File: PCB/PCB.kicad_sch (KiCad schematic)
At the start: 3 parts, among them J1 TFT Display, J2 PowerBoost 500c, U1 Pico

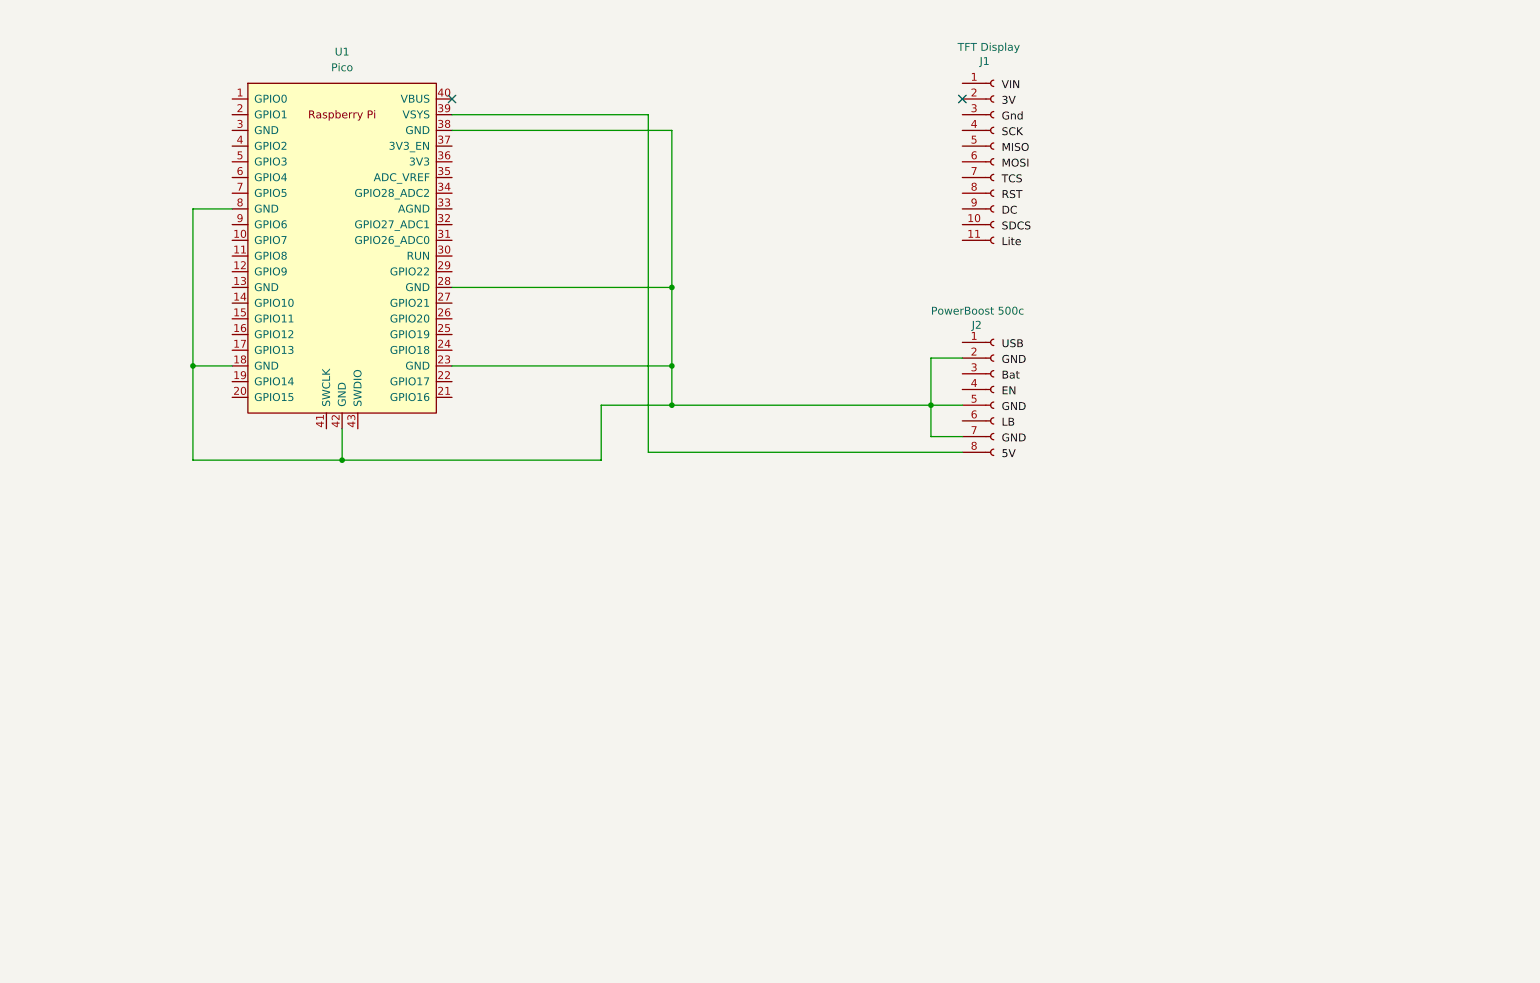
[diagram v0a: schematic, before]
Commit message: Finished controller schematic and mostly finished pcb
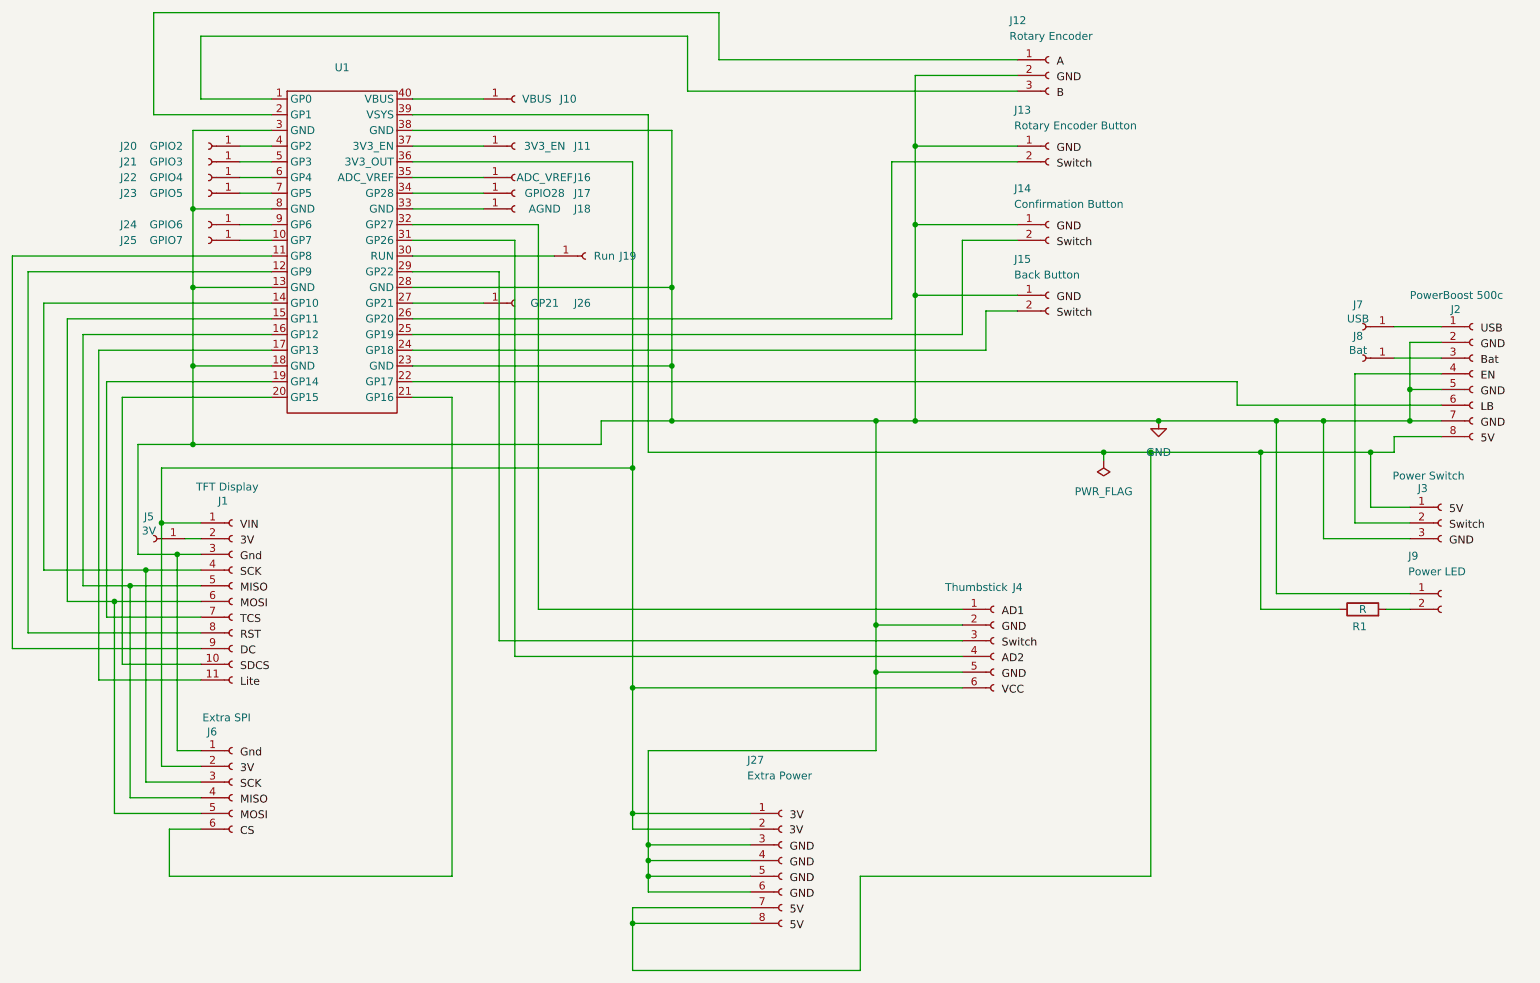
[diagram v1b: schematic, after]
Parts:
- removed U1: Pico, RPi_Pico:RPi_Pico_SMD_TH, symbol RPi_Pico:Pico
- added J10: VBUS, Connector_PinHeader_2.54mm:PinHeader_1x01_P2.54mm_Vertical, symbol Connector:Conn_01x01_Socket
- added J11: 3V3_EN, Connector_PinHeader_2.54mm:PinHeader_1x01_P2.54mm_Vertical, symbol Connector:Conn_01x01_Socket
- added J12: Rotary Encoder, Connector_PinHeader_2.54mm:PinHeader_1x03_P2.54mm_Vertical, symbol Connector:Conn_01x03_Socket
- added J13: Rotary Encoder Button, Connector_PinHeader_2.54mm:PinHeader_1x02_P2.54mm_Vertical, symbol Connector:Conn_01x02_Socket
- added J14: Confirmation Button, Connector_PinHeader_2.54mm:PinHeader_1x02_P2.54mm_Vertical, symbol Connector:Conn_01x02_Socket
- added J15: Back Button, Connector_PinHeader_2.54mm:PinHeader_1x02_P2.54mm_Vertical, symbol Connector:Conn_01x02_Socket
- added J16: ADC_VREF, Connector_PinHeader_2.54mm:PinHeader_1x01_P2.54mm_Vertical, symbol Connector:Conn_01x01_Socket
- added J17: GPIO28, Connector_PinHeader_2.54mm:PinHeader_1x01_P2.54mm_Vertical, symbol Connector:Conn_01x01_Socket
- added J18: AGND, Connector_PinHeader_2.54mm:PinHeader_1x01_P2.54mm_Vertical, symbol Connector:Conn_01x01_Socket
- added J19: Run, Connector_PinHeader_2.54mm:PinHeader_1x01_P2.54mm_Vertical, symbol Connector:Conn_01x01_Socket
- added J20: GPIO2, Connector_PinHeader_2.54mm:PinHeader_1x01_P2.54mm_Vertical, symbol Connector:Conn_01x01_Socket
- added J21: GPIO3, Connector_PinHeader_2.54mm:PinHeader_1x01_P2.54mm_Vertical, symbol Connector:Conn_01x01_Socket
- added J22: GPIO4, Connector_PinHeader_2.54mm:PinHeader_1x01_P2.54mm_Vertical, symbol Connector:Conn_01x01_Socket
- added J23: GPIO5, Connector_PinHeader_2.54mm:PinHeader_1x01_P2.54mm_Vertical, symbol Connector:Conn_01x01_Socket
- added J24: GPIO6, Connector_PinHeader_2.54mm:PinHeader_1x01_P2.54mm_Vertical, symbol Connector:Conn_01x01_Socket
- added J25: GPIO7, Connector_PinHeader_2.54mm:PinHeader_1x01_P2.54mm_Vertical, symbol Connector:Conn_01x01_Socket
- added J26: GP21, Connector_PinHeader_2.54mm:PinHeader_1x01_P2.54mm_Vertical, symbol Connector:Conn_01x01_Socket
- added J27: Extra Power, Connector_PinHeader_2.54mm:PinHeader_1x08_P2.54mm_Vertical, symbol Connector:Conn_01x08_Socket
- added J3: Power Switch, Connector_PinHeader_2.54mm:PinHeader_1x03_P2.54mm_Vertical, symbol Connector:Conn_01x03_Socket
- added J4: Thumbstick, Connector_PinHeader_2.54mm:PinHeader_1x06_P2.54mm_Vertical, symbol Connector:Conn_01x06_Socket
- added J5: 3V, Connector_PinHeader_2.54mm:PinHeader_1x01_P2.54mm_Vertical, symbol Connector:Conn_01x01_Socket
- added J6: Extra SPI, Connector_PinHeader_2.54mm:PinHeader_1x06_P2.54mm_Vertical, symbol Connector:Conn_01x06_Socket
- added J7: USB, Connector_PinHeader_2.54mm:PinHeader_1x01_P2.54mm_Vertical, symbol Connector:Conn_01x01_Socket
- added J8: Bat, Connector_PinHeader_2.54mm:PinHeader_1x01_P2.54mm_Vertical, symbol Connector:Conn_01x01_Socket
- added J9: Power LED, Connector_PinHeader_2.54mm:PinHeader_1x02_P2.54mm_Vertical, symbol Connector:Conn_01x02_Socket
- added R1: R, Resistor_THT:R_Axial_DIN0204_L3.6mm_D1.6mm_P5.08mm_Horizontal, symbol Device:R
- added U1: ~, SuperyardageLib:RasPi_Pico, symbol SuperyardageLib:RasPi_Pico
- J1: footprint (none) -> Connector_PinHeader_2.54mm:PinHeader_1x11_P2.54mm_Vertical
- J2: footprint (none) -> Connector_PinHeader_2.54mm:PinHeader_1x08_P2.54mm_Vertical
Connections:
- net GND: now also J1.3 (Pin_3), J2.2 (Pin_2), J2.5 (Pin_5), J2.7 (Pin_7), J12.2 (Pin_2), J13.1 (Pin_1), J14.1 (Pin_1), J15.1 (Pin_1), J27.3 (Pin_3), J27.4 (Pin_4), J27.5 (Pin_5), J27.6 (Pin_6), J3.3 (Pin_3), J4.2 (Pin_2), J4.5 (Pin_5), J6.1 (Pin_1), J9.1 (Pin_1), U1.13 (GND), U1.18 (GND), U1.23 (GND), U1.28 (GND), U1.3 (GND), U1.38 (GND), U1.8 (GND)
- net at J2.8 (Pin_8): now also J27.7 (Pin_7), J27.8 (Pin_8), J3.1 (Pin_1), R1.1, U1.39 (VSYS)
- net at J1.1 (Pin_1): now also J27.1 (Pin_1), J27.2 (Pin_2), J4.6 (Pin_6), J6.2 (Pin_2), U1.36 (3V3_OUT)
- net at J1.10 (Pin_10): now also U1.20 (GP15)
- net at J1.11 (Pin_11): now also U1.17 (GP13)
- net at J1.2 (Pin_2): now also J5.1 (Pin_1)
- net at J1.4 (Pin_4): now also J6.3 (Pin_3), U1.14 (GP10)
- net at J1.5 (Pin_5): now also J6.4 (Pin_4), U1.16 (GP12)
- net at J1.6 (Pin_6): now also J6.5 (Pin_5), U1.15 (GP11)
- net at J1.7 (Pin_7): now also U1.19 (GP14)
- net at J1.8 (Pin_8): now also U1.12 (GP9)
- net at J1.9 (Pin_9): now also U1.11 (GP8)
- net at J2.1 (Pin_1): now also J7.1 (Pin_1)
- net at J2.3 (Pin_3): now also J8.1 (Pin_1)
- net at J2.4 (Pin_4): now also J3.2 (Pin_2)
- net at J2.6 (Pin_6): now also U1.22 (GP17)
- new net: J13.2 (Pin_2), U1.26 (GP20)
- new net: J10.1 (Pin_1), U1.40 (VBUS)
- new net: J4.1 (Pin_1), U1.32 (GP27)
- new net: J4.3 (Pin_3), U1.29 (GP22)
- new net: J4.4 (Pin_4), U1.31 (GP26)
- new net: J11.1 (Pin_1), U1.37 (3V3_EN)
- new net: J21.1 (Pin_1), U1.5 (GP3)
- new net: J20.1 (Pin_1), U1.4 (GP2)
- new net: J26.1 (Pin_1), U1.27 (GP21)
- new net: J9.2 (Pin_2), R1.2
- new net: J16.1 (Pin_1), U1.35 (ADC_VREF)
- new net: J12.1 (Pin_1), U1.2 (GP1)
- new net: J12.3 (Pin_3), U1.1 (GP0)
- new net: J6.6 (Pin_6), U1.21 (GP16)
- new net: J25.1 (Pin_1), U1.10 (GP7)
- new net: J23.1 (Pin_1), U1.7 (GP5)
- new net: J14.2 (Pin_2), U1.25 (GP19)
- new net: J17.1 (Pin_1), U1.34 (GP28)
- new net: J19.1 (Pin_1), U1.30 (RUN)
- new net: J24.1 (Pin_1), U1.9 (GP6)
- new net: J15.2 (Pin_2), U1.24 (GP18)
- new net: J18.1 (Pin_1), U1.33 (GND)
- new net: J22.1 (Pin_1), U1.6 (GP4)
- no-connect marks 2 -> 0
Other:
- moved on the sheet: J1, J2
